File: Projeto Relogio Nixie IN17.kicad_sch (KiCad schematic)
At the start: 64 parts, among them J1 Conn_01x04, J2 Conn_01x24, J3 Conn_01x24, J4 BATTERY, J5 ANTENNA, Q1 BC817, Q2 STD17NF25, Q3 BC817, Q4 BC548, Q5 BC548, Q6 BC548, SW1 SW_Push, SW2 SW_Push, SW3 SPST_B3U-1000P, SW4 SPST_B3U-1000P, U1 MAX1771xSA, U2 CP2102N-A01-GQFN24, U3 HV5523K7-G, U4 PAM2305AABADJ, U5 MCP73831-3-OT, U6 ESP32-PICO-D4

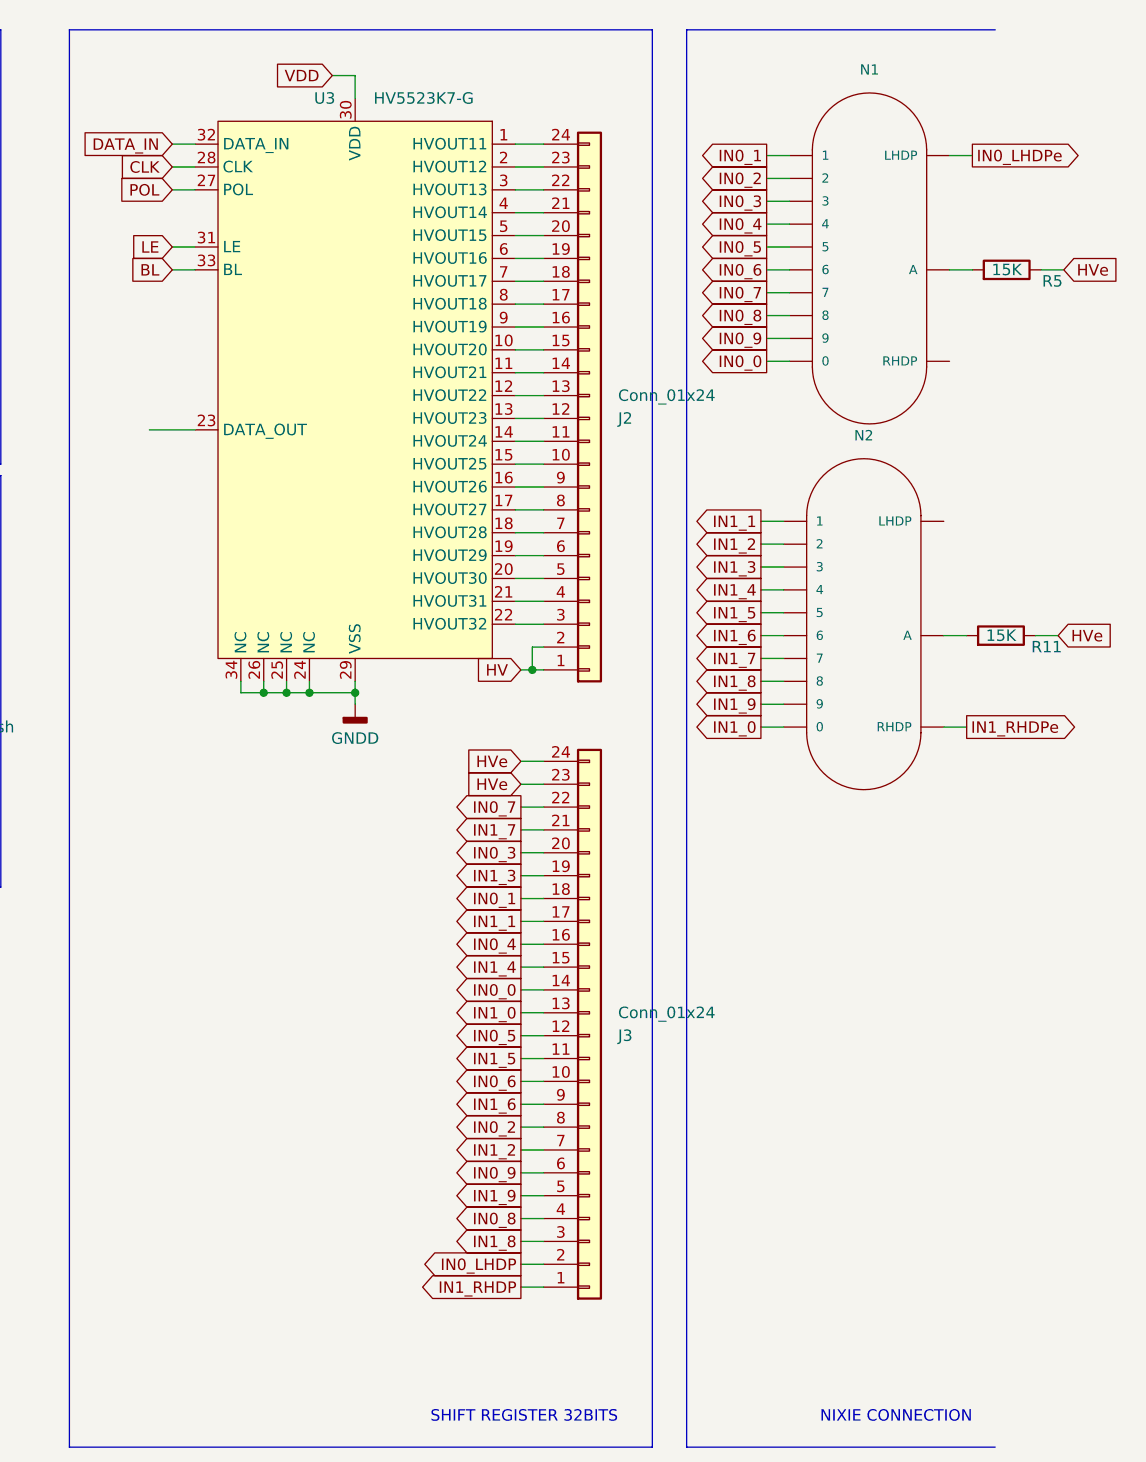
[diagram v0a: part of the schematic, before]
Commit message: Add files via upload
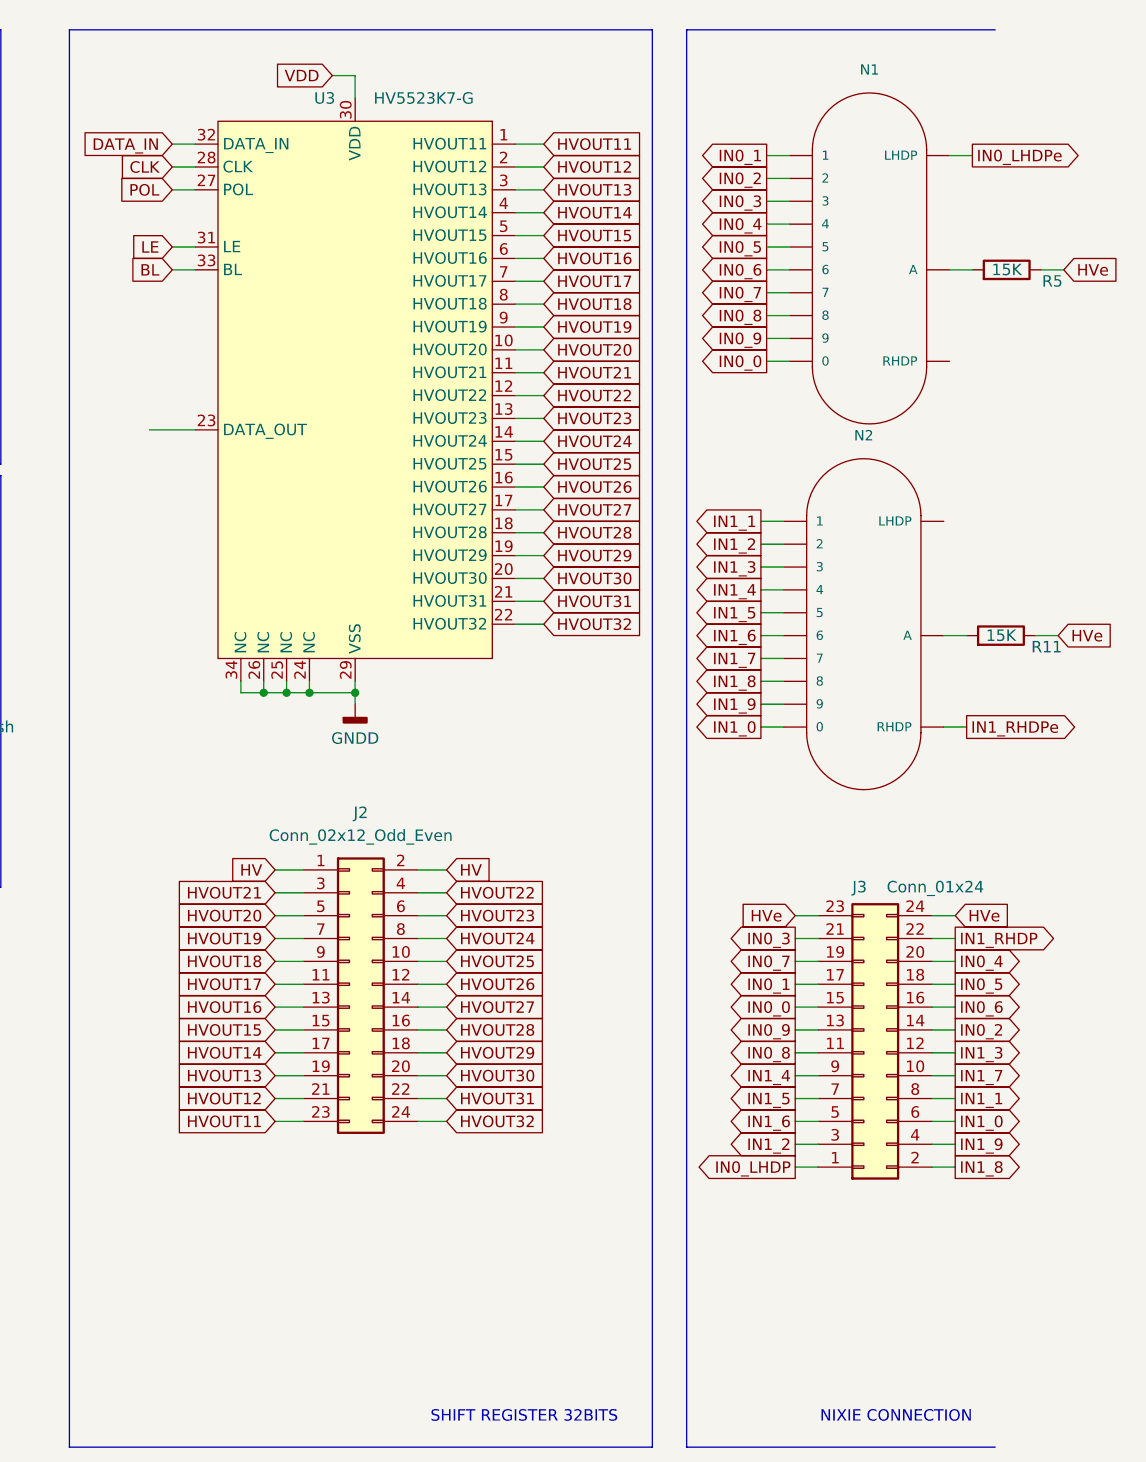
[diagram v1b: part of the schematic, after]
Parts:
- removed J2: Conn_01x24, Connector_PinHeader_1.27mm:PinHeader_2x12_P1.27mm_Vertical, symbol Connector_Generic:Conn_01x24
- added J2: Conn_02x12_Odd_Even, Connector_PinHeader_1.27mm:PinHeader_2x12_P1.27mm_Vertical, symbol Connector_Generic:Conn_02x12_Odd_Even
- J3: symbol Connector_Generic:Conn_01x24 -> Connector_Generic:Conn_02x12_Odd_Even
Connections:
- net HV: now also J2.1 (Pin_1), J2.2 (Pin_2)
- net IN0_0: now also J3.15 (Pin_15); no longer J3.14 (Pin_14)
- net IN0_1: now also J3.17 (Pin_17); no longer J3.18 (Pin_18)
- net IN0_2: now also J3.14 (Pin_14); no longer J3.8 (Pin_8)
- net IN0_3: now also J3.21 (Pin_21); no longer J3.20 (Pin_20)
- net IN0_4: now also J3.20 (Pin_20); no longer J3.16 (Pin_16)
- net IN0_5: now also J3.18 (Pin_18); no longer J3.12 (Pin_12)
- net IN0_6: now also J3.16 (Pin_16); no longer J3.10 (Pin_10)
- net IN0_7: now also J3.19 (Pin_19); no longer J3.22 (Pin_22)
- net IN0_8: now also J3.11 (Pin_11); no longer J3.4 (Pin_4)
- net IN0_9: now also J3.13 (Pin_13); no longer J3.6 (Pin_6)
- net IN0_LHDP: now also J3.1 (Pin_1); no longer J3.2 (Pin_2)
- net IN1_0: now also J3.6 (Pin_6); no longer J3.13 (Pin_13)
- net IN1_1: now also J3.8 (Pin_8); no longer J3.17 (Pin_17)
- net IN1_2: now also J3.3 (Pin_3); no longer J3.7 (Pin_7)
- net IN1_3: now also J3.12 (Pin_12); no longer J3.19 (Pin_19)
- net IN1_4: now also J3.9 (Pin_9); no longer J3.15 (Pin_15)
- net IN1_5: now also J3.7 (Pin_7); no longer J3.11 (Pin_11)
- net IN1_6: now also J3.5 (Pin_5); no longer J3.9 (Pin_9)
- net IN1_7: now also J3.10 (Pin_10); no longer J3.21 (Pin_21)
- net IN1_8: now also J3.2 (Pin_2); no longer J3.3 (Pin_3)
- net IN1_9: now also J3.4 (Pin_4); no longer J3.5 (Pin_5)
- net IN1_RHDP: now also J3.22 (Pin_22); no longer J3.1 (Pin_1)
- net HVOUT11: now reaches U3.1 (HVOUT11)
- net HVOUT11: now also J2.23 (Pin_23)
- net HVOUT20: now reaches U3.10 (HVOUT20)
- net HVOUT20: now also J2.5 (Pin_5)
- net HVOUT21: now reaches U3.11 (HVOUT21)
- net HVOUT21: now also J2.3 (Pin_3)
- net HVOUT22: now reaches U3.12 (HVOUT22)
- net HVOUT22: now also J2.4 (Pin_4)
- net HVOUT23: now reaches U3.13 (HVOUT23)
- net HVOUT23: now also J2.6 (Pin_6)
- net HVOUT24: now reaches U3.14 (HVOUT24)
- net HVOUT24: now also J2.8 (Pin_8)
- net HVOUT25: now reaches U3.15 (HVOUT25)
- net HVOUT25: now also J2.10 (Pin_10)
- net HVOUT26: now reaches U3.16 (HVOUT26)
- net HVOUT26: now also J2.12 (Pin_12)
- net HVOUT27: now reaches U3.17 (HVOUT27)
- net HVOUT27: now also J2.14 (Pin_14)
- net HVOUT28: now reaches U3.18 (HVOUT28)
- net HVOUT28: now also J2.16 (Pin_16)
- net HVOUT29: now reaches U3.19 (HVOUT29)
- net HVOUT29: now also J2.18 (Pin_18)
- net HVOUT12: now reaches U3.2 (HVOUT12)
- net HVOUT12: now also J2.21 (Pin_21)
- net HVOUT30: now reaches U3.20 (HVOUT30)
- net HVOUT30: now also J2.20 (Pin_20)
- net HVOUT31: now reaches U3.21 (HVOUT31)
- net HVOUT31: now also J2.22 (Pin_22)
- net HVOUT32: now reaches U3.22 (HVOUT32)
- net HVOUT32: now also J2.24 (Pin_24)
- net HVOUT13: now reaches U3.3 (HVOUT13)
- net HVOUT13: now also J2.19 (Pin_19)
- net HVOUT14: now reaches U3.4 (HVOUT14)
- net HVOUT14: now also J2.17 (Pin_17)
- net HVOUT15: now reaches U3.5 (HVOUT15)
- net HVOUT15: now also J2.15 (Pin_15)
- net HVOUT16: now reaches U3.6 (HVOUT16)
- net HVOUT16: now also J2.13 (Pin_13)
- net HVOUT17: now reaches U3.7 (HVOUT17)
- net HVOUT17: now also J2.11 (Pin_11)
- net HVOUT18: now reaches U3.8 (HVOUT18)
- net HVOUT18: now also J2.9 (Pin_9)
- net HVOUT19: now reaches U3.9 (HVOUT19)
- net HVOUT19: now also J2.7 (Pin_7)
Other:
- moved on the sheet: J3

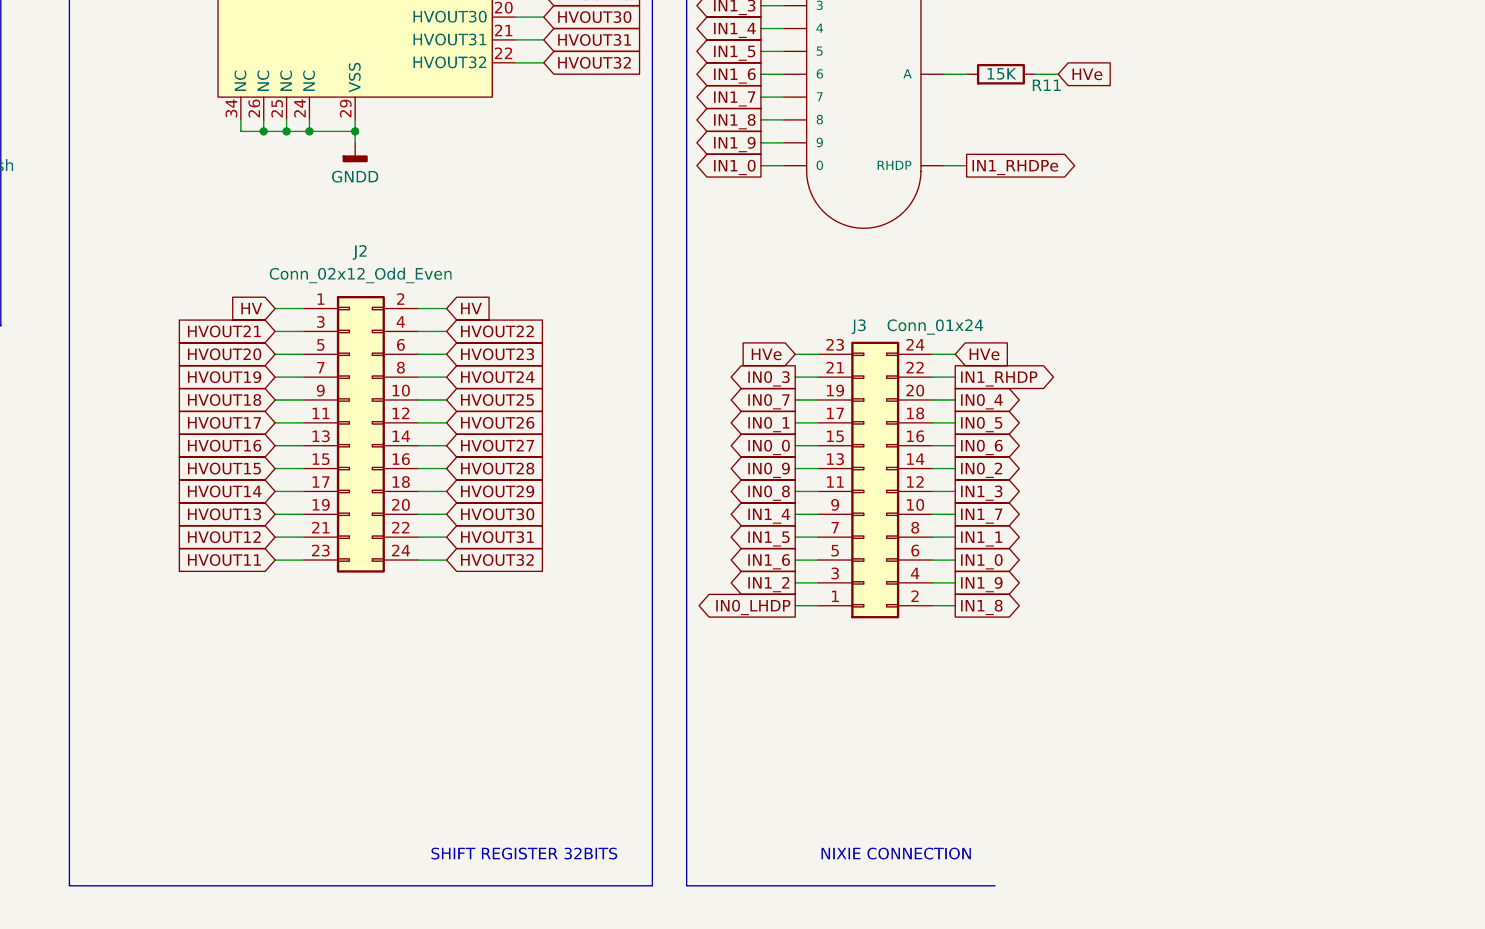
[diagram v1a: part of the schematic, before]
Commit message: Add files via upload
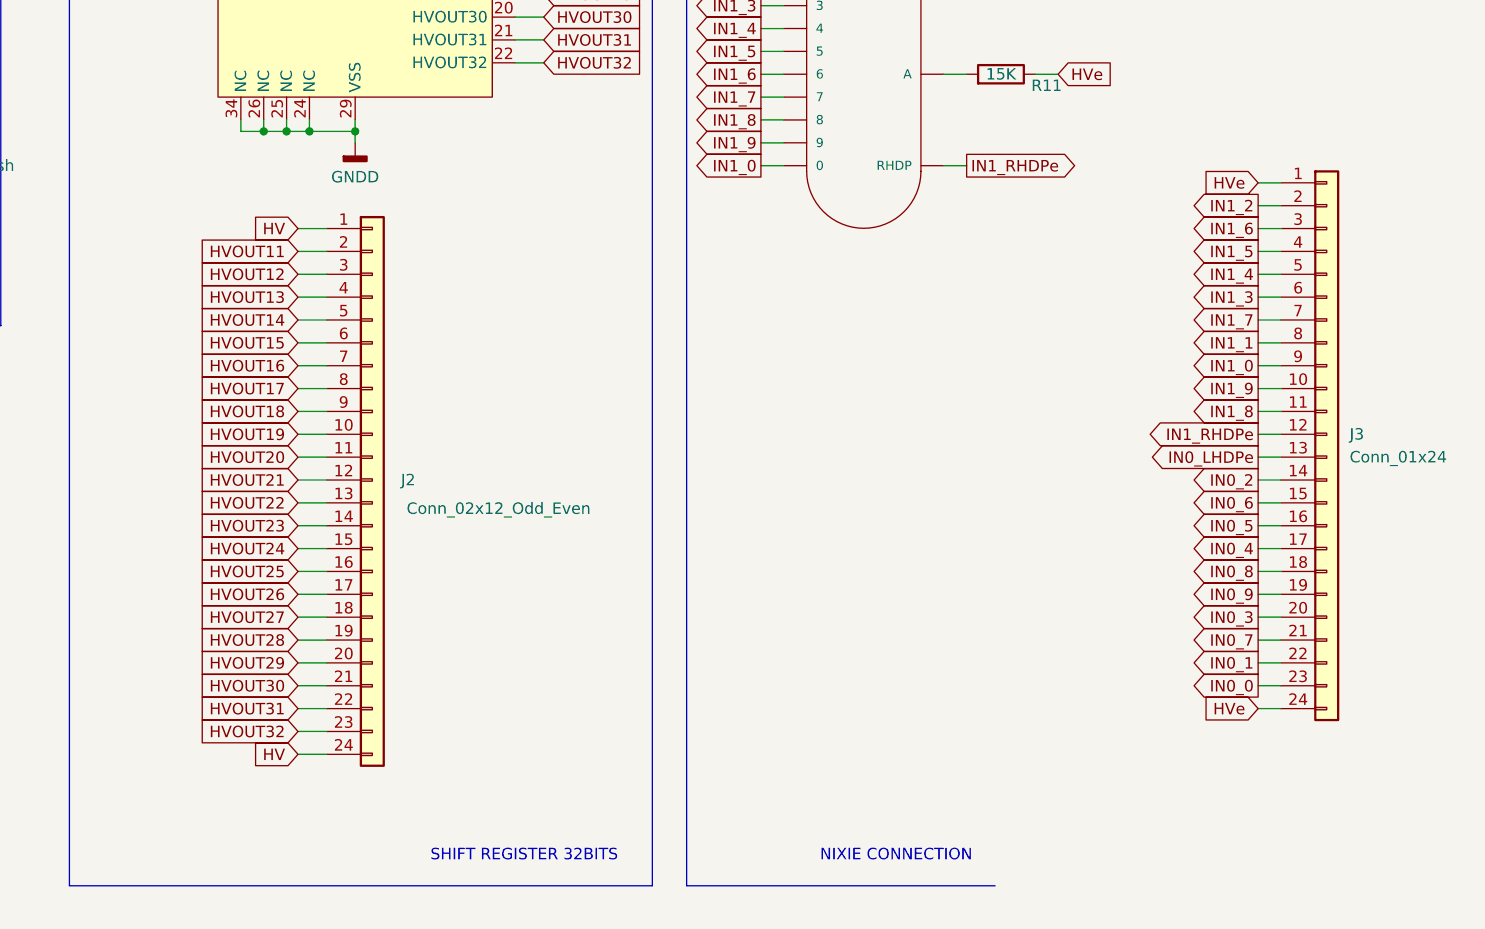
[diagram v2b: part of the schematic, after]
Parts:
- removed J3: Conn_01x24, Connector_PinHeader_1.27mm:PinHeader_2x12_P1.27mm_Vertical, symbol Connector_Generic:Conn_02x12_Odd_Even
- added J3: Conn_01x24, Connector_FFC-FPC:TE_2-1734839-4_1x24-1MP_P0.5mm_Horizontal, symbol Connector_Generic:Conn_01x24
- J2: footprint Connector_PinHeader_1.27mm:PinHeader_2x12_P1.27mm_Vertical -> Connector_FFC-FPC:TE_2-1734839-4_1x24-1MP_P0.5mm_Horizontal; symbol Connector_Generic:Conn_02x12_Odd_Even -> Connector_Generic:Conn_01x24
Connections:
- net HV: now also J2.24 (Pin_24); no longer J2.2 (Pin_2)
- net HVOUT11: now also J2.2 (Pin_2); no longer J2.23 (Pin_23)
- net HVOUT12: now also J2.3 (Pin_3); no longer J2.21 (Pin_21)
- net HVOUT13: now also J2.4 (Pin_4); no longer J2.19 (Pin_19)
- net HVOUT14: now also J2.5 (Pin_5); no longer J2.17 (Pin_17)
- net HVOUT15: now also J2.6 (Pin_6); no longer J2.15 (Pin_15)
- net HVOUT16: now also J2.7 (Pin_7); no longer J2.13 (Pin_13)
- net HVOUT17: now also J2.8 (Pin_8); no longer J2.11 (Pin_11)
- net HVOUT19: now also J2.10 (Pin_10); no longer J2.7 (Pin_7)
- net HVOUT20: now also J2.11 (Pin_11); no longer J2.5 (Pin_5)
- net HVOUT21: now also J2.12 (Pin_12); no longer J2.3 (Pin_3)
- net HVOUT22: now also J2.13 (Pin_13); no longer J2.4 (Pin_4)
- net HVOUT23: now also J2.14 (Pin_14); no longer J2.6 (Pin_6)
- net HVOUT24: now also J2.15 (Pin_15); no longer J2.8 (Pin_8)
- net HVOUT25: now also J2.16 (Pin_16); no longer J2.10 (Pin_10)
- net HVOUT26: now also J2.17 (Pin_17); no longer J2.12 (Pin_12)
- net HVOUT27: now also J2.18 (Pin_18); no longer J2.14 (Pin_14)
- net HVOUT28: now also J2.19 (Pin_19); no longer J2.16 (Pin_16)
- net HVOUT29: now also J2.20 (Pin_20); no longer J2.18 (Pin_18)
- net HVOUT30: now also J2.21 (Pin_21); no longer J2.20 (Pin_20)
- net HVOUT32: now also J2.23 (Pin_23); no longer J2.24 (Pin_24)
- net HVe: now also J3.1 (Pin_1), J3.24 (Pin_24)
- net IN0_0: now also J3.23 (Pin_23)
- net IN0_1: now also J3.22 (Pin_22)
- net IN0_2: now also J3.14 (Pin_14)
- net IN0_3: now also J3.20 (Pin_20)
- net IN0_4: now also J3.17 (Pin_17)
- net IN0_5: now also J3.16 (Pin_16)
- net IN0_6: now also J3.15 (Pin_15)
- net IN0_7: now also J3.21 (Pin_21)
- net IN0_8: now also J3.18 (Pin_18)
- net IN0_9: now also J3.19 (Pin_19)
- net IN0_LHDPe: now also J3.13 (Pin_13)
- net IN1_0: now also J3.9 (Pin_9)
- net IN1_1: now also J3.8 (Pin_8)
- net IN1_2: now also J3.2 (Pin_2)
- net IN1_3: now also J3.6 (Pin_6)
- net IN1_4: now also J3.5 (Pin_5)
- net IN1_5: now also J3.4 (Pin_4)
- net IN1_6: now also J3.3 (Pin_3)
- net IN1_7: now also J3.7 (Pin_7)
- net IN1_8: now also J3.11 (Pin_11)
- net IN1_9: now also J3.10 (Pin_10)
- net IN1_RHDPe: now also J3.12 (Pin_12)
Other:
- moved on the sheet: J2
